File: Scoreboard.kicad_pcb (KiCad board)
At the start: 2 copper layers, 140.5 x 64.5 mm, 256 parts, among them J1 TC2050-IDC-NL, P1 USB_C_Plug_USB2.0, Q1 HL-2301V, Q10 HL-2302V, Q11 HL-2302V, Q12 HL-2302V, Q13 HL-2302V, Q14 HL-2302V, Q15 HL-2302V, Q16 HL-2302V, Q17 HL-2302V, Q18 HL-2302V, Q19 HL-2302V, Q2 HL-2301V, Q20 HL-2302V, Q21 HL-2302V, Q22 HL-2302V, Q23 HL-2302V, Q24 HL-2302V, Q25 HL-2302V, Q3 HL-2301V, Q4 HL-2301V, Q5 HL-2301V, Q6 HL-2301V, Q7 HL-2301V, Q8 HL-2302V, Q9 HL-2302V, SW2 SW_Push, SW3 SW_Push, SW4 SW_Push, U1 AP63203WU, U2 BM832, U3 LM66100DCKR, U4 LM66100DCKR

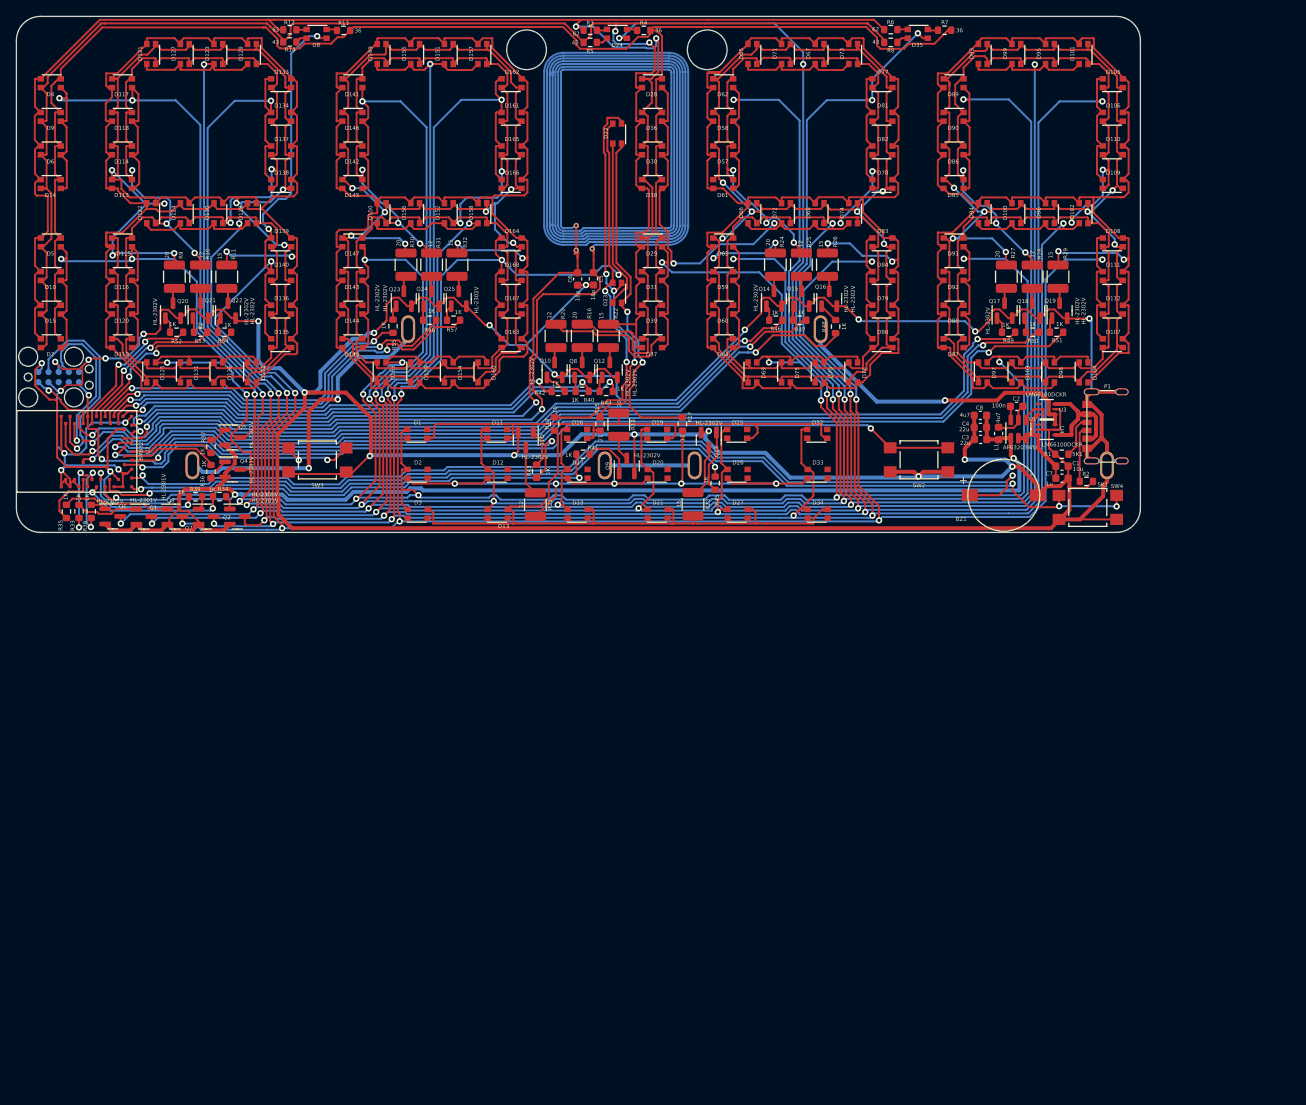
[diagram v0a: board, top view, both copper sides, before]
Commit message: Made a new hardware revision
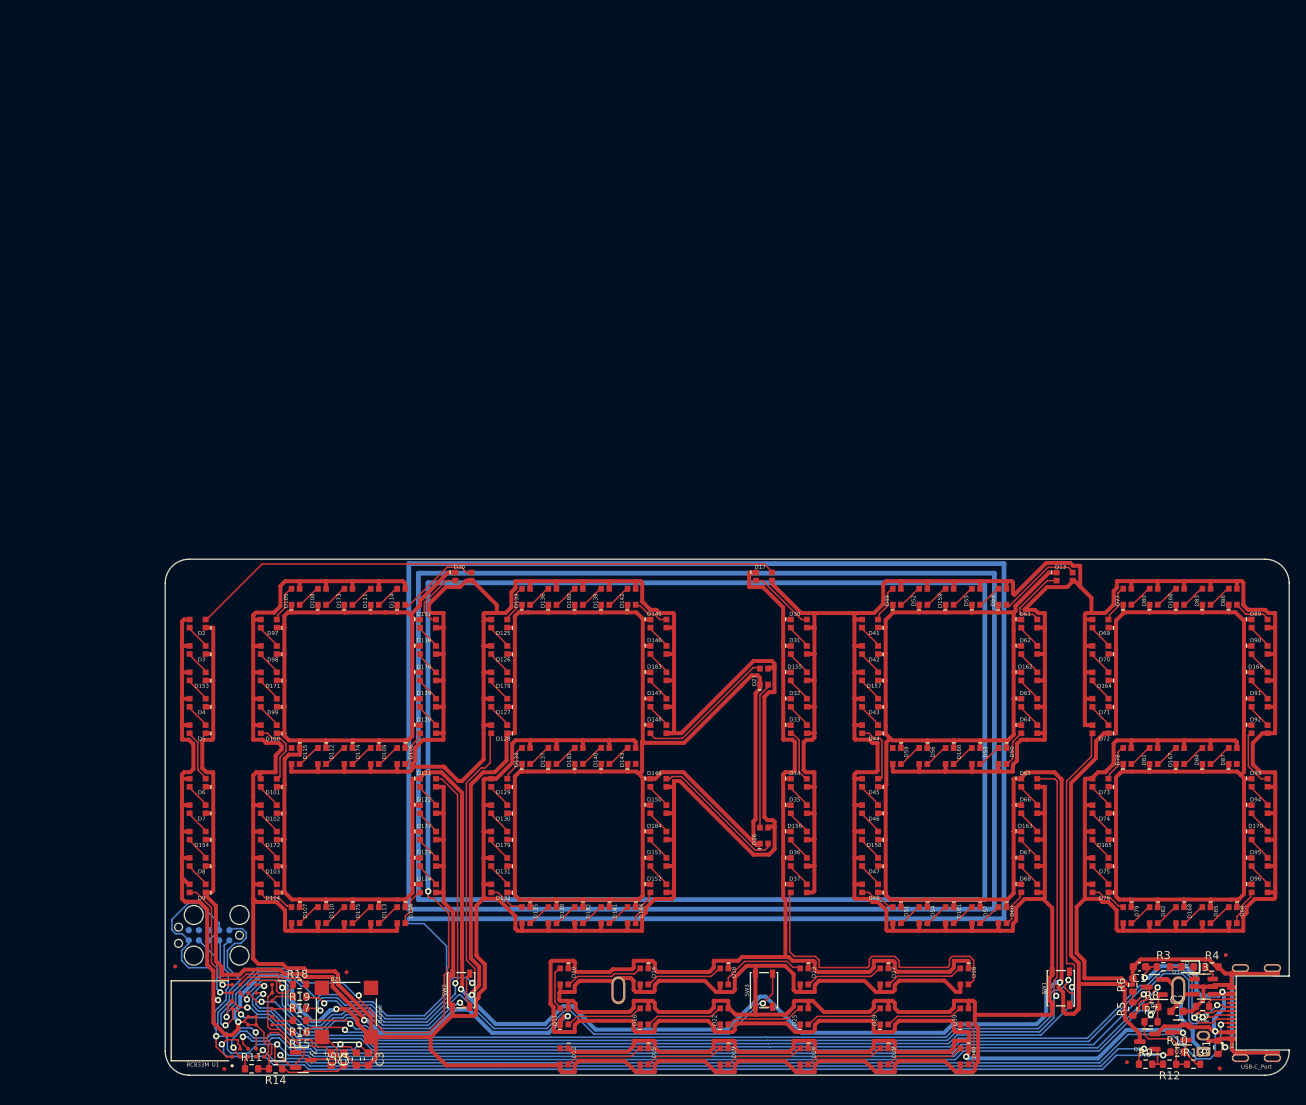
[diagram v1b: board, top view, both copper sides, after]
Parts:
- removed BT3: AA_BATTERY, User_Footprints:BAT_BCAAPC
- removed the C2 at (191.0, 78.2)
- removed C7: 1u, Capacitor_SMD:C_0603_1608Metric
- removed C8: 4u7, Capacitor_SMD:C_0603_1608Metric
- removed the D12 at (126.2, 86.6)
- removed the D30 at (145.4, 46.1)
- removed the D6 at (70.3, 46.1)
- removed L1: 4u7, Inductor_SMD:L_0603_1608Metric
- removed P1: USB_C_Plug_USB2.0, User_Footprints:DEALON_USB-TYPE-C-009
- removed Q10, Q11, Q12, Q13, Q14, Q15, Q16, Q17, Q18, Q19, Q20, Q21, Q22, Q23, Q24, Q25, Q8, Q9: HL-2302V, Package_TO_SOT_SMD:SOT-23
- removed Q5, Q6, Q7: HL-2301V, Package_TO_SOT_SMD:SOT-23
- removed R20, R21, R25, R28, R31: 12, Resistor_SMD:R_1210_3225Metric
- removed R22, R23, R26, R29, R32: 15, Resistor_SMD:R_1210_3225Metric
- removed R24, R27, R30: 20, Resistor_SMD:R_1210_3225Metric
- removed R33, R34, R35, R36, R37, R38, R39, R40, R41, R42, R43, R44, R45, R46, R47, R48, R49, R50, R51, R52, R53, R54, R55, R56, R57: 1K, Resistor_SMD:R_0603_1608Metric
- removed SW4: SW_Push, User_Footprints:SW_SPST_TSC015A03526A
- removed U2: BM832, User_Footprints:BM832
- removed U3, U4: LM66100DCKR, User_Footprints:DCK6_TEX-L
- added D169: LED_WS2812B, User_Footprints:LED_WS2812B_2x1.8mm, F.Cu at (221.4, 111.9)
- added D170: LED_WS2812B, User_Footprints:LED_WS2812B_2x1.8mm, F.Cu at (221.4, 131.8)
- added D171: LED_WS2812B, User_Footprints:LED_WS2812B_2x1.8mm, F.Cu at (97.5, 111.9)
- added D172: LED_WS2812B, User_Footprints:LED_WS2812B_2x1.8mm, F.Cu at (97.5, 131.8)
- added D173: LED_WS2812B, User_Footprints:LED_WS2812B_2x1.8mm, F.Cu at (107.5, 102.0)
- added D174: LED_WS2812B, User_Footprints:LED_WS2812B_2x1.8mm, F.Cu at (107.5, 121.8)
- added D175: LED_WS2812B, User_Footprints:LED_WS2812B_2x1.8mm, F.Cu at (107.5, 141.7)
- added D176: LED_WS2812B, User_Footprints:LED_WS2812B_2x1.8mm, F.Cu at (117.4, 111.9)
- added D177: LED_WS2812B, User_Footprints:LED_WS2812B_2x1.8mm, F.Cu at (117.5, 131.8)
- added D178: LED_WS2812B, User_Footprints:LED_WS2812B_2x1.8mm, F.Cu at (126.4, 111.9)
- added D179: LED_WS2812B, User_Footprints:LED_WS2812B_2x1.8mm, F.Cu at (126.4, 131.8)
- added D180: LED_WS2812B, User_Footprints:LED_WS2812B_2x1.8mm, F.Cu at (136.3, 102.0)
- added D181: LED_WS2812B, User_Footprints:LED_WS2812B_2x1.8mm, F.Cu at (136.3, 121.8)
- added D182: LED_WS2812B, User_Footprints:LED_WS2812B_2x1.8mm, F.Cu at (136.3, 141.7)
- added D183: LED_WS2812B, User_Footprints:LED_WS2812B_2x1.8mm, F.Cu at (146.3, 111.9)
- added D184: LED_WS2812B, User_Footprints:LED_WS2812B_2x1.8mm, F.Cu at (146.2, 131.8)
- added D37: LED_WS2812B, User_Footprints:LED_WS2812B_2x1.8mm, F.Cu at (163.8, 138.4)
- added D40: LED_WS2812B, User_Footprints:LED_WS2812B_2x1.8mm, F.Cu at (184.5, 159.4)
- added D41: LED_WS2812B, User_Footprints:LED_WS2812B_2x1.8mm, F.Cu at (172.7, 105.3)
- added D42: LED_WS2812B, User_Footprints:LED_WS2812B_2x1.8mm, F.Cu at (172.7, 108.6)
- added D43: LED_WS2812B, User_Footprints:LED_WS2812B_2x1.8mm, F.Cu at (172.7, 115.2)
- added D44: LED_WS2812B, User_Footprints:LED_WS2812B_2x1.8mm, F.Cu at (172.7, 118.5)
- added D45: LED_WS2812B, User_Footprints:LED_WS2812B_2x1.8mm, F.Cu at (172.7, 125.2)
- added D46: LED_WS2812B, User_Footprints:LED_WS2812B_2x1.8mm, F.Cu at (172.7, 128.5)
- added D47: LED_WS2812B, User_Footprints:LED_WS2812B_2x1.8mm, F.Cu at (172.7, 135.1)
- added D48: LED_WS2812B, User_Footprints:LED_WS2812B_2x1.8mm, F.Cu at (172.7, 138.4)
- added D49: LED_WS2812B, User_Footprints:LED_WS2812B_2x1.8mm, F.Cu at (176.1, 101.9)
- added D50: LED_WS2812B, User_Footprints:LED_WS2812B_2x1.8mm, F.Cu at (189.2, 121.8)
- added D51: LED_WS2812B, User_Footprints:LED_WS2812B_2x1.8mm, F.Cu at (176.1, 141.7)
- added D52: LED_WS2812B, User_Footprints:LED_WS2812B_2x1.8mm, F.Cu at (179.4, 101.9)
- added D53: LED_WS2812B, User_Footprints:LED_WS2812B_2x1.8mm, F.Cu at (185.9, 121.8)
- added D54: LED_WS2812B, User_Footprints:LED_WS2812B_2x1.8mm, F.Cu at (179.4, 141.7)
- added D55: LED_WS2812B, User_Footprints:LED_WS2812B_2x1.8mm, F.Cu at (186.0, 101.9)
- added D56: LED_WS2812B, User_Footprints:LED_WS2812B_2x1.8mm, F.Cu at (179.3, 121.8)
- added D62: LED_WS2812B, User_Footprints:LED_WS2812B_2x1.8mm, F.Cu at (192.6, 108.6)
- added D69: LED_WS2812B, User_Footprints:LED_WS2812B_2x1.8mm, F.Cu at (201.5, 105.3)
- added D90: LED_WS2812B, User_Footprints:LED_WS2812B_2x1.8mm, F.Cu at (221.4, 108.6)
- added J2: USB-C_Port, User_Footprints:GCT_USB4110GFA, F.Cu at (219.0, 154.0)
- added J3: TP4057, User_Footprints:SOT-23-6, F.Cu at (214.4, 150.7)
- added REF**: Fiducial_0.5mm_Mask1mm, Fiducial:Fiducial_0.5mm_Mask1mm, F.Cu at (92.0, 161.0)
- added REF**: Fiducial_0.5mm_Mask1mm, Fiducial:Fiducial_0.5mm_Mask1mm, F.Cu at (85.8, 148.2)
- added REF**: Fiducial_0.5mm_Mask1mm, Fiducial:Fiducial_0.5mm_Mask1mm, F.Cu at (204.8, 160.1)
- added REF**: Fiducial_0.5mm_Mask1mm, Fiducial:Fiducial_0.5mm_Mask1mm, F.Cu at (107.3, 148.9)
- added REF**: Fiducial_0.5mm_Mask1mm, Fiducial:Fiducial_0.5mm_Mask1mm, F.Cu at (216.4, 160.9)
- added REF**: Fiducial_0.5mm_Mask1mm, Fiducial:Fiducial_0.5mm_Mask1mm, F.Cu at (217.2, 146.7)
- added SW1: SW_Push, User_Footprints:Oval_Button, F.Cu at (196.6, 150.9)
- AE1: footprint User_Footprints:HM-NFC-Class6-Antenna -> User_Footprints:HM-NFC-Class3-Antenna
- BT1: value AA_BATTERY -> LiPo; footprint User_Footprints:BAT_BCAAPC -> User_Footprints:JST_PH_S2B-PH-K_1x02_P2.00mm_Horizontal
- BT2: value AA_BATTERY -> 18650_Cell; footprint User_Footprints:BAT_BCAAPC -> User_Footprints:18650_Cell_Holder
- BZ1: value HYG-9032A -> Buzzer; footprint User_Footprints:MagneticBuzzer_HYG-9032A -> User_Footprints:XDCR_CMT-7525-80-SMT-TR
- C1: value 10u -> 1u; footprint Capacitor_SMD:C_0603_1608Metric -> User_Footprints:C_0603_1608Metric
- C2: renamed from D37; value LED_RGAB -> 1u; footprint User_Footprints:RGB_LED_NH-B2020RGBA-HF -> User_Footprints:C_0603_1608Metric
- C3, C4: value 22u -> 18p; footprint Capacitor_SMD:C_0603_1608Metric -> User_Footprints:C_0603_1608Metric
- C5, C6: value 18p -> 4u7; footprint Capacitor_SMD:C_0603_1608Metric -> User_Footprints:C_0603_1608Metric
- D1: value LED_RGAB -> LED; footprint User_Footprints:RGB_LED_NH-B2020RGBA-HF -> LED_SMD:LED_0603_1608Metric
- D10, D100, D101, D102, D103, D104, D105, D106, D107, D108, D109, D11, D110, D111, D112, D113, D114, D115, D116, D117, D118, D119, D120, D121, D122, D123, D124, D125, D126, D127, D128, D129, D13, D130, D131, D132, D133, D134, D135, D136, D137, D138, D139, D14, D140, D141, D142, D143, D144, D145, D146, D147, D148, D149, D15, D150, D151, D152, D153, D154, D155, D156, D157, D158, D159, D16, D160, D161, D162, D163, D164, D165, D166, D167, D168, D17, D18, D19, D2, D20, D21, D22, D23, D24, D25, D26, D27, D28, D29, D3, D31, D32, D33, D34, D35, D36, D38, D39, D4, D5, D57, D58, D59, D60, D61, D63, D64, D65, D66, D67, D68, D7, D70, D71, D72, D73, D74, D75, D76, D77, D78, D79, D8, D80, D81, D82, D83, D84, D85, D86, D87, D88, D89, D9, D91, D92, D93, D94, D95, D96, D97, D98, D99: value LED_RGAB -> LED_WS2812B; footprint User_Footprints:RGB_LED_NH-B2020RGBA-HF -> User_Footprints:LED_WS2812B_2x1.8mm
- D12: renamed from D69; value LED_RGAB -> LED_WS2812B; footprint User_Footprints:RGB_LED_NH-B2020RGBA-HF -> User_Footprints:LED_WS2812B_2x1.8mm
- D30: renamed from D90; value LED_RGAB -> LED_WS2812B; footprint User_Footprints:RGB_LED_NH-B2020RGBA-HF -> User_Footprints:LED_WS2812B_2x1.8mm
- D6: renamed from D62; value LED_RGAB -> LED_WS2812B; footprint User_Footprints:RGB_LED_NH-B2020RGBA-HF -> User_Footprints:LED_WS2812B_2x1.8mm
- Q1, Q2, Q3, Q4: footprint Package_TO_SOT_SMD:SOT-23 -> User_Footprints:SOT-23
- R1, R2: footprint Resistor_SMD:R_0603_1608Metric -> User_Footprints:R_0603_1608Metric
- R10: value 12 -> 1K; footprint Resistor_SMD:R_1210_3225Metric -> User_Footprints:R_0603_1608Metric
- R11: value 15 -> 1K; footprint Resistor_SMD:R_1210_3225Metric -> User_Footprints:R_0603_1608Metric
- R12: value 62 -> 100K; footprint Resistor_SMD:R_0603_1608Metric -> User_Footprints:R_0603_1608Metric
- R13, R7: value 36 -> 100K; footprint Resistor_SMD:R_0603_1608Metric -> User_Footprints:R_0603_1608Metric
- R14: value 43 -> 100K; footprint Resistor_SMD:R_0603_1608Metric -> User_Footprints:R_0603_1608Metric
- R15: value 21 -> 1K; footprint Resistor_SMD:R_0603_1608Metric -> User_Footprints:R_0603_1608Metric
- R16, R18, R9: value 20 -> 1K; footprint Resistor_SMD:R_1210_3225Metric -> User_Footprints:R_0603_1608Metric
- R17: value 12 -> 1K; footprint Resistor_SMD:R_0603_1608Metric -> User_Footprints:R_0603_1608Metric
- R19: value 15 -> 1K; footprint Resistor_SMD:R_0603_1608Metric -> User_Footprints:R_0603_1608Metric
- R3: value 62 -> 1K; footprint Resistor_SMD:R_0603_1608Metric -> User_Footprints:R_0603_1608Metric
- R4: value 36 -> 1K6; footprint Resistor_SMD:R_0603_1608Metric -> User_Footprints:R_0603_1608Metric
- R5: value 43 -> 5K1; footprint Resistor_SMD:R_0603_1608Metric -> User_Footprints:R_0603_1608Metric
- R6: value 62 -> 5K1; footprint Resistor_SMD:R_0603_1608Metric -> User_Footprints:R_0603_1608Metric
- R8: value 43 -> 1K; footprint Resistor_SMD:R_0603_1608Metric -> User_Footprints:R_0603_1608Metric
- SW2, SW3: footprint User_Footprints:SW_SPST_TSC015A03526A -> User_Footprints:Oval_Button
- U1: value AP63203WU -> BC833M; footprint Package_TO_SOT_SMD:TSOT-23-6 -> User_Footprints:XCVR_BC833M
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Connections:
- BZ1 pad 1: Net-(U2-PadP$17) -> Net-(BZ1-Pad1)
- C1 pad 1: Net-(C1-Pad1) -> VBUS
- C2 pad 1: RED_BOTT_2 -> VBAT
- C2 pad 2: GREEN_BOTT_2 -> GND
- C3 pad 1: +3V3 -> Net-(AE1-Pad1)
- C4 pad 1: +3V3 -> GND
- C4 pad 2: GND -> Net-(AE1-Pad2)
- C5 pad 1: GND -> VBUS
- C5 pad 2: Net-(AE1-Pad2) -> GND
- C6 pad 1: Net-(AE1-Pad1) -> VDD
- D1 pad 1: RED_BOTT_1 -> Net-(D1-Pad1)
- D1 pad 2: unconnected-(D1-Pad2) -> Net-(D1-Pad2)
- D10 pad 1: RED_BOTT_2 -> VLEDS_E
- D10 pad 2: GREEN_BOTT_2 -> Net-(D10-Pad2)
- D10 pad 3: Segment_2-E_OUT -> GND
- D10 pad 4: BLUE_BOTT_2 -> Net-(D10-Pad4)
- D100 pad 1: RED_RIGHT_2 -> VLEDS
- D100 pad 2: GREEN_RIGHT_2 -> Net-(D100-Pad2)
- D100 pad 3: Segment_2-G_OUT -> GND
- D100 pad 4: BLUE_RIGHT_2 -> Net-(D100-Pad4)
- D101 pad 1: RED_RIGHT_2 -> VLEDS
- D101 pad 2: GREEN_RIGHT_2 -> Net-(D100-Pad4)
- D101 pad 3: Segment_2-A_OUT -> GND
- D101 pad 4: BLUE_RIGHT_2 -> Net-(D101-Pad4)
- D102 pad 1: RED_RIGHT_2 -> VLEDS
- D102 pad 2: GREEN_RIGHT_2 -> Net-(D101-Pad4)
- D102 pad 3: Segment_2-G_OUT -> GND
- D102 pad 4: BLUE_RIGHT_2 -> Net-(D102-Pad4)
- D103 pad 1: RED_RIGHT_2 -> VLEDS
- D103 pad 2: GREEN_RIGHT_2 -> Net-(D103-Pad2)
- D103 pad 3: Segment_2-D_OUT -> GND
- D103 pad 4: BLUE_RIGHT_2 -> Net-(D103-Pad4)
- D104 pad 1: RED_RIGHT_2 -> VLEDS
- D104 pad 2: GREEN_RIGHT_2 -> Net-(D103-Pad4)
- D104 pad 3: Segment_2-D_OUT -> GND
- D104 pad 4: BLUE_RIGHT_2 -> Net-(D104-Pad4)
- D105 pad 1: RED_RIGHT_2 -> VLEDS
- D105 pad 2: GREEN_RIGHT_2 -> Net-(D105-Pad2)
- D105 pad 3: Segment_2-B_OUT -> GND
- D105 pad 4: BLUE_RIGHT_2 -> Net-(D105-Pad4)
- D106 pad 1: RED_RIGHT_2 -> VLEDS
- D106 pad 2: GREEN_RIGHT_2 -> Net-(D106-Pad2)
- D106 pad 3: Segment_2-B_OUT -> GND
- D106 pad 4: BLUE_RIGHT_2 -> Net-(D106-Pad4)
- D107 pad 1: RED_RIGHT_2 -> VLEDS
- D107 pad 2: GREEN_RIGHT_2 -> Net-(D104-Pad4)
- D107 pad 3: Segment_2-C_OUT -> GND
- D107 pad 4: BLUE_RIGHT_2 -> Net-(D107-Pad4)
- D108 pad 1: RED_RIGHT_2 -> VLEDS
- D108 pad 2: GREEN_RIGHT_2 -> Net-(D108-Pad2)
- D108 pad 3: Segment_2-C_OUT -> GND
- D108 pad 4: BLUE_RIGHT_2 -> Net-(D105-Pad2)
- D109 pad 1: RED_RIGHT_2 -> VLEDS
- D109 pad 2: GREEN_RIGHT_2 -> Net-(D109-Pad2)
- D109 pad 3: Segment_2-B_OUT -> GND
- D109 pad 4: BLUE_RIGHT_2 -> Net-(D106-Pad2)
- D11 pad 1: RED_BOTT_1 -> VLEDS_E
- D11 pad 2: unconnected-(D11-Pad2) -> Net-(D11-Pad2)
- D11 pad 3: Segment_2-E_OUT -> GND
- D11 pad 4: unconnected-(D11-Pad4) -> Net-(D10-Pad2)
- D110 pad 1: RED_RIGHT_2 -> VLEDS
- D110 pad 2: GREEN_RIGHT_2 -> Net-(D107-Pad4)
- D110 pad 3: Segment_2-B_OUT -> GND
- D110 pad 4: BLUE_RIGHT_2 -> Net-(D110-Pad4)
- D111 pad 1: RED_RIGHT_2 -> VLEDS
- D111 pad 2: GREEN_RIGHT_2 -> Net-(D111-Pad2)
- D111 pad 3: Segment_2-C_OUT -> GND
- D111 pad 4: BLUE_RIGHT_2 -> Net-(D111-Pad4)
- D112 pad 1: RED_RIGHT_2 -> VLEDS
- D112 pad 2: GREEN_RIGHT_2 -> Net-(D112-Pad2)
- D112 pad 3: Segment_2-C_OUT -> GND
- D112 pad 4: BLUE_RIGHT_2 -> Net-(D112-Pad4)
- D113 pad 1: RED_LEFT_1 -> VLEDS
- D113 pad 2: GREEN_LEFT_1 -> Net-(D113-Pad2)
- D113 pad 3: Segment_2-F_OUT -> GND
- D113 pad 4: BLUE_LEFT_1 -> Net-(D113-Pad4)
- D114 pad 1: RED_LEFT_1 -> VLEDS
- D114 pad 2: GREEN_LEFT_1 -> Net-(D114-Pad2)
- D114 pad 3: Segment_2-F_OUT -> GND
- D114 pad 4: BLUE_LEFT_1 -> Net-(D111-Pad2)
- D115 pad 1: RED_LEFT_1 -> VLEDS
- D115 pad 2: GREEN_LEFT_1 -> unconnected-(D115-Pad2)
- D115 pad 3: Segment_2-E_OUT -> GND
- D115 pad 4: BLUE_LEFT_1 -> Net-(D112-Pad2)
- D116 pad 1: RED_LEFT_1 -> VLEDS
- D116 pad 2: GREEN_LEFT_1 -> Net-(D113-Pad4)
- D116 pad 3: Segment_2-E_OUT -> GND
- D116 pad 4: BLUE_LEFT_1 -> Net-(D116-Pad4)
- D117 pad 1: RED_LEFT_1 -> VLEDS
- D117 pad 2: GREEN_LEFT_1 -> Net-(D117-Pad2)
- D117 pad 3: Segment_2-F_OUT -> GND
- D117 pad 4: BLUE_LEFT_1 -> Net-(D117-Pad4)
- D118 pad 1: RED_LEFT_1 -> VLEDS
- D118 pad 2: GREEN_LEFT_1 -> Net-(D118-Pad2)
- D118 pad 3: Segment_2-F_OUT -> GND
- D118 pad 4: BLUE_LEFT_1 -> Net-(D117-Pad2)
- D119 pad 1: RED_LEFT_1 -> VLEDS
- D119 pad 2: GREEN_LEFT_1 -> Net-(D119-Pad2)
- D119 pad 3: Segment_2-E_OUT -> GND
- D119 pad 4: BLUE_LEFT_1 -> Net-(D119-Pad4)
- D12 pad 1: RED_RIGHT_1 -> VLEDS_E
- D12 pad 2: GREEN_RIGHT_1 -> unconnected-(D12-Pad2)
- D12 pad 3: Segment_2-D_OUT -> GND
- D12 pad 4: BLUE_RIGHT_1 -> Net-(D12-Pad4)
- D120 pad 1: RED_LEFT_1 -> VLEDS
- D120 pad 2: GREEN_LEFT_1 -> Net-(D106-Pad4)
- D120 pad 3: Segment_2-E_OUT -> GND
- D120 pad 4: BLUE_LEFT_1 -> Net-(D119-Pad2)
- D121 pad 1: RED_LEFT_1 -> VLEDS
- D121 pad 2: GREEN_LEFT_1 -> Net-(D121-Pad2)
- D121 pad 3: Segment_2-A_OUT -> GND
- D121 pad 4: BLUE_LEFT_1 -> L1_Data
- D122 pad 1: RED_LEFT_1 -> VLEDS
- D122 pad 2: GREEN_LEFT_1 -> Net-(D122-Pad2)
- D122 pad 3: Segment_2-G_OUT -> GND
- D122 pad 4: BLUE_LEFT_1 -> Net-(D121-Pad2)
- D123 pad 1: RED_LEFT_1 -> VLEDS
- D123 pad 2: GREEN_LEFT_1 -> Net-(D123-Pad2)
- D123 pad 3: Segment_2-A_OUT -> GND
- D123 pad 4: BLUE_LEFT_1 -> Net-(D123-Pad4)
- D124 pad 1: RED_LEFT_1 -> VLEDS
- D124 pad 2: GREEN_LEFT_1 -> Net-(D116-Pad4)
- D124 pad 3: Segment_2-G_OUT -> GND
- D124 pad 4: BLUE_LEFT_1 -> Net-(D123-Pad2)
- D125 pad 1: RED_LEFT_1 -> VLEDS
- D125 pad 2: GREEN_LEFT_1 -> Net-(D125-Pad2)
- D125 pad 3: Segment_2-D_OUT -> GND
- D125 pad 4: BLUE_LEFT_1 -> Net-(D125-Pad4)
- D126 pad 1: RED_LEFT_1 -> VLEDS
- D126 pad 2: GREEN_LEFT_1 -> Net-(D125-Pad4)
- D126 pad 3: Segment_2-D_OUT -> GND
- D126 pad 4: BLUE_LEFT_1 -> Net-(D126-Pad4)
- D127 pad 1: RED_LEFT_1 -> VLEDS
- D127 pad 2: GREEN_LEFT_1 -> Net-(D127-Pad2)
- D127 pad 3: Segment_2-A_OUT -> GND
- D127 pad 4: BLUE_LEFT_1 -> Net-(D127-Pad4)
- D128 pad 1: RED_LEFT_1 -> VLEDS
- D128 pad 2: GREEN_LEFT_1 -> Net-(D127-Pad4)
- D128 pad 3: Segment_2-G_OUT -> GND
- D128 pad 4: BLUE_LEFT_1 -> L2_Data
- D129 pad 1: RED_LEFT_1 -> VLEDS
- D129 pad 2: GREEN_LEFT_1 -> Net-(D129-Pad2)
- D129 pad 3: Segment_2-A_OUT -> GND
- D129 pad 4: BLUE_LEFT_1 -> Net-(D129-Pad4)
- D13 pad 1: unconnected-(D13-Pad1) -> VLEDS
- D13 pad 2: unconnected-(D13-Pad2) -> Net-(D13-Pad2)
- D13 pad 3: Segment_2-E_OUT -> GND
- D13 pad 4: BLUE_BOTT_1 -> Net-(D13-Pad4)
- D130 pad 1: RED_LEFT_1 -> VLEDS
- D130 pad 2: GREEN_LEFT_1 -> Net-(D129-Pad4)
- D130 pad 3: Segment_2-G_OUT -> GND
- D130 pad 4: BLUE_LEFT_1 -> Net-(D130-Pad4)
- D131 pad 1: RED_LEFT_1 -> VLEDS
- D131 pad 2: GREEN_LEFT_1 -> Net-(D131-Pad2)
- D131 pad 3: Segment_2-D_OUT -> GND
- D131 pad 4: BLUE_LEFT_1 -> Net-(D131-Pad4)
- D132 pad 1: RED_LEFT_1 -> VLEDS
- D132 pad 2: GREEN_LEFT_1 -> Net-(D131-Pad4)
- D132 pad 3: Segment_2-D_OUT -> GND
- D132 pad 4: BLUE_LEFT_1 -> Net-(D132-Pad4)
- D133 pad 1: RED_LEFT_1 -> VLEDS
- D133 pad 2: GREEN_LEFT_1 -> Net-(D133-Pad2)
- D133 pad 3: Segment_2-B_OUT -> GND
- D133 pad 4: BLUE_LEFT_1 -> Net-(D125-Pad2)
- D134 pad 1: RED_LEFT_1 -> VLEDS
- D134 pad 2: GREEN_LEFT_1 -> Net-(D134-Pad2)
- D134 pad 3: Segment_2-B_OUT -> GND
- D134 pad 4: BLUE_LEFT_1 -> Net-(D129-Pad2)
- D135 pad 1: RED_LEFT_1 -> VLEDS
- D135 pad 2: GREEN_LEFT_1 -> Net-(D132-Pad4)
- D135 pad 3: Segment_2-C_OUT -> GND
- D135 pad 4: BLUE_LEFT_1 -> Net-(D135-Pad4)
- D136 pad 1: RED_LEFT_1 -> VLEDS
- D136 pad 2: GREEN_LEFT_1 -> Net-(D136-Pad2)
- D136 pad 3: Segment_2-C_OUT -> GND
- D136 pad 4: BLUE_LEFT_1 -> Net-(D133-Pad2)
- D137 pad 1: RED_LEFT_1 -> VLEDS
- D137 pad 2: GREEN_LEFT_1 -> Net-(D137-Pad2)
- D137 pad 3: Segment_2-B_OUT -> GND
- D137 pad 4: BLUE_LEFT_1 -> Net-(D134-Pad2)
- D138 pad 1: RED_LEFT_1 -> VLEDS
- D138 pad 2: GREEN_LEFT_1 -> Net-(D135-Pad4)
- D138 pad 3: Segment_2-B_OUT -> GND
- D138 pad 4: BLUE_LEFT_1 -> Net-(D138-Pad4)
- D139 pad 1: RED_LEFT_1 -> VLEDS
- D139 pad 2: GREEN_LEFT_1 -> Net-(D139-Pad2)
- D139 pad 3: Segment_2-C_OUT -> GND
- D139 pad 4: BLUE_LEFT_1 -> Net-(D139-Pad4)
- D14 pad 1: RED_BOTT_2 -> VLEDS_E
- D14 pad 2: GREEN_BOTT_2 -> Net-(D10-Pad4)
- D14 pad 3: Segment_2-F_OUT -> GND
- D14 pad 4: BLUE_BOTT_2 -> Net-(D14-Pad4)
- D140 pad 1: RED_LEFT_1 -> VLEDS
- D140 pad 2: GREEN_LEFT_1 -> Net-(D140-Pad2)
- D140 pad 3: Segment_2-C_OUT -> GND
- D140 pad 4: BLUE_LEFT_1 -> Net-(D140-Pad4)
- D141 pad 1: RED_LEFT_2 -> VLEDS
- D141 pad 2: GREEN_LEFT_2 -> Net-(D141-Pad2)
- D141 pad 3: Segment_2-F_OUT -> GND
- D141 pad 4: BLUE_LEFT_2 -> Net-(D141-Pad4)
- D142 pad 1: RED_LEFT_2 -> VLEDS
- D142 pad 2: GREEN_LEFT_2 -> Net-(D142-Pad2)
- D142 pad 3: Segment_2-F_OUT -> GND
- D142 pad 4: BLUE_LEFT_2 -> Net-(D139-Pad2)
- D143 pad 1: RED_LEFT_2 -> VLEDS
- D143 pad 2: GREEN_LEFT_2 -> unconnected-(D143-Pad2)
- D143 pad 3: Segment_2-E_OUT -> GND
- D143 pad 4: BLUE_LEFT_2 -> Net-(D140-Pad2)
- D144 pad 1: RED_LEFT_2 -> VLEDS
- D144 pad 2: GREEN_LEFT_2 -> Net-(D141-Pad4)
- D144 pad 3: Segment_2-E_OUT -> GND
- D144 pad 4: BLUE_LEFT_2 -> Net-(D144-Pad4)
- D145 pad 1: RED_LEFT_2 -> VLEDS
- D145 pad 2: GREEN_LEFT_2 -> Net-(D145-Pad2)
- D145 pad 3: Segment_2-F_OUT -> GND
- D145 pad 4: BLUE_LEFT_2 -> Net-(D142-Pad2)
- D146 pad 1: RED_LEFT_2 -> VLEDS
- D146 pad 2: GREEN_LEFT_2 -> Net-(D146-Pad2)
- D146 pad 3: Segment_2-F_OUT -> GND
- D146 pad 4: BLUE_LEFT_2 -> Net-(D145-Pad2)
- D147 pad 1: RED_LEFT_2 -> VLEDS
- D147 pad 2: GREEN_LEFT_2 -> Net-(D147-Pad2)
- D147 pad 3: Segment_2-E_OUT -> GND
- D147 pad 4: BLUE_LEFT_2 -> Net-(D147-Pad4)
- D148 pad 1: RED_LEFT_2 -> VLEDS
- D148 pad 2: GREEN_LEFT_2 -> Net-(D148-Pad2)
- D148 pad 3: Segment_2-E_OUT -> GND
- D148 pad 4: BLUE_LEFT_2 -> Net-(D147-Pad2)
- D149 pad 1: RED_LEFT_2 -> VLEDS
- D149 pad 2: GREEN_LEFT_2 -> Net-(D149-Pad2)
- D149 pad 3: Segment_2-A_OUT -> GND
- D149 pad 4: BLUE_LEFT_2 -> Net-(D149-Pad4)
- D15 pad 1: RED_BOTT_2 -> VLEDS_E
- D15 pad 2: GREEN_BOTT_2 -> Net-(D12-Pad4)
- D15 pad 3: Segment_2-E_OUT -> GND
- D15 pad 4: BLUE_BOTT_2 -> Net-(D15-Pad4)
- D150 pad 1: RED_LEFT_2 -> VLEDS
- D150 pad 2: GREEN_LEFT_2 -> Net-(D150-Pad2)
- D150 pad 3: Segment_2-G_OUT -> GND
- D150 pad 4: BLUE_LEFT_2 -> Net-(D149-Pad2)
- D151 pad 1: RED_LEFT_2 -> VLEDS
- D151 pad 2: GREEN_LEFT_2 -> Net-(D151-Pad2)
- D151 pad 3: Segment_2-A_OUT -> GND
- D151 pad 4: BLUE_LEFT_2 -> Net-(D151-Pad4)
- D152 pad 1: RED_LEFT_2 -> VLEDS
- D152 pad 2: GREEN_LEFT_2 -> Net-(D144-Pad4)
- D152 pad 3: Segment_2-G_OUT -> GND
- D152 pad 4: BLUE_LEFT_2 -> Net-(D151-Pad2)
- D153 pad 1: RED_LEFT_2 -> VLEDS_E
- D153 pad 2: GREEN_LEFT_2 -> Net-(D153-Pad2)
- D153 pad 3: Segment_2-D_OUT -> GND
- D153 pad 4: BLUE_LEFT_2 -> Net-(D153-Pad4)
- D154 pad 1: RED_LEFT_2 -> VLEDS_E
- D154 pad 2: GREEN_LEFT_2 -> Net-(D154-Pad2)
- D154 pad 3: Segment_2-D_OUT -> GND
- D154 pad 4: BLUE_LEFT_2 -> Net-(D154-Pad4)
- D155 pad 1: RED_LEFT_2 -> VLEDS_E
- D155 pad 2: GREEN_LEFT_2 -> Net-(D155-Pad2)
- D155 pad 3: Segment_2-A_OUT -> GND
- D155 pad 4: BLUE_LEFT_2 -> Net-(D155-Pad4)
- D156 pad 1: RED_LEFT_2 -> VLEDS_E
- D156 pad 2: GREEN_LEFT_2 -> Net-(D156-Pad2)
- D156 pad 3: Segment_2-G_OUT -> GND
- D156 pad 4: BLUE_LEFT_2 -> Net-(D156-Pad4)
- D157 pad 1: RED_LEFT_2 -> VLEDS
- D157 pad 2: GREEN_LEFT_2 -> Net-(D157-Pad2)
- D157 pad 3: Segment_2-A_OUT -> GND
- D157 pad 4: BLUE_LEFT_2 -> Net-(D157-Pad4)
- D158 pad 1: RED_LEFT_2 -> VLEDS
- D158 pad 2: GREEN_LEFT_2 -> Net-(D158-Pad2)
- D158 pad 3: Segment_2-G_OUT -> GND
- D158 pad 4: BLUE_LEFT_2 -> Net-(D158-Pad4)
- D159 pad 1: RED_LEFT_2 -> VLEDS
- D159 pad 2: GREEN_LEFT_2 -> Net-(D159-Pad2)
- D159 pad 3: Segment_2-D_OUT -> GND
- D159 pad 4: BLUE_LEFT_2 -> Net-(D159-Pad4)
- D16 pad 1: RED_BOTT_1 -> VLEDS_E
- D16 pad 2: unconnected-(D16-Pad2) -> Net-(D16-Pad2)
- D16 pad 3: Segment_2-F_OUT -> GND
- D16 pad 4: unconnected-(D16-Pad4) -> Net-(D11-Pad2)
- D160 pad 1: RED_LEFT_2 -> VLEDS
- D160 pad 2: GREEN_LEFT_2 -> Net-(D160-Pad2)
- D160 pad 3: Segment_2-D_OUT -> GND
- D160 pad 4: BLUE_LEFT_2 -> Net-(D160-Pad4)
- D161 pad 1: RED_LEFT_2 -> VLEDS
- D161 pad 2: GREEN_LEFT_2 -> Net-(D161-Pad2)
- D161 pad 3: Segment_2-B_OUT -> GND
- D161 pad 4: BLUE_LEFT_2 -> Net-(D161-Pad4)
- D162 pad 1: RED_LEFT_2 -> VLEDS
- D162 pad 2: GREEN_LEFT_2 -> Net-(D162-Pad2)
- D162 pad 3: Segment_2-B_OUT -> GND
- D162 pad 4: BLUE_LEFT_2 -> Net-(D162-Pad4)
- D163 pad 1: RED_LEFT_2 -> VLEDS
- D163 pad 2: GREEN_LEFT_2 -> Net-(D163-Pad2)
- D163 pad 3: Segment_2-C_OUT -> GND
- D163 pad 4: BLUE_LEFT_2 -> Net-(D163-Pad4)
- D164 pad 1: RED_LEFT_2 -> VLEDS
- D164 pad 2: GREEN_LEFT_2 -> Net-(D164-Pad2)
- D164 pad 3: Segment_2-C_OUT -> GND
- D164 pad 4: BLUE_LEFT_2 -> Net-(D164-Pad4)
- D165 pad 1: RED_LEFT_2 -> VLEDS
- D165 pad 2: GREEN_LEFT_2 -> Net-(D165-Pad2)
- D165 pad 3: Segment_2-B_OUT -> GND
- D165 pad 4: BLUE_LEFT_2 -> Net-(D165-Pad4)
- D166 pad 1: RED_LEFT_2 -> VLEDS
- D166 pad 2: GREEN_LEFT_2 -> Net-(D166-Pad2)
- D166 pad 3: Segment_2-B_OUT -> GND
- D166 pad 4: BLUE_LEFT_2 -> Net-(D166-Pad4)
- D167 pad 1: RED_LEFT_2 -> VLEDS
- D167 pad 2: GREEN_LEFT_2 -> Net-(D167-Pad2)
- D167 pad 3: Segment_2-C_OUT -> GND
- D167 pad 4: BLUE_LEFT_2 -> Net-(D167-Pad4)
- D168 pad 1: RED_LEFT_2 -> VLEDS
- D168 pad 2: GREEN_LEFT_2 -> Net-(D168-Pad2)
- D168 pad 3: Segment_2-C_OUT -> GND
- D168 pad 4: BLUE_LEFT_2 -> Net-(D168-Pad4)
- D17 pad 1: unconnected-(D17-Pad1) -> VLEDS_E
- D17 pad 2: GREEN_BOTT_1 -> Net-(D17-Pad2)
- D17 pad 3: Segment_2-F_OUT -> GND
- D17 pad 4: unconnected-(D17-Pad4) -> Net-(D17-Pad4)
- D18 pad 1: unconnected-(D18-Pad1) -> VLEDS_E
- D18 pad 2: unconnected-(D18-Pad2) -> Net-(D14-Pad4)
- D18 pad 3: Segment_2-F_OUT -> GND
- D18 pad 4: BLUE_BOTT_1 -> Net-(D18-Pad4)
- D19 pad 1: RED_BOTT_1 -> VLEDS_E
- D19 pad 2: unconnected-(D19-Pad2) -> Net-(D15-Pad4)
- D19 pad 3: Segment_2-A_OUT -> GND
- D19 pad 4: unconnected-(D19-Pad4) -> Net-(D19-Pad4)
- D2 pad 1: unconnected-(D2-Pad1) -> VLEDS_E
- D2 pad 2: GREEN_BOTT_1 -> Net-(D17-Pad4)
- D2 pad 3: Segment_2-D_OUT -> GND
- D2 pad 4: unconnected-(D2-Pad4) -> Net-(D2-Pad4)
- D20 pad 1: unconnected-(D20-Pad1) -> VLEDS
- D20 pad 2: GREEN_BOTT_1 -> Net-(D117-Pad4)
- D20 pad 3: Segment_2-A_OUT -> GND
- D20 pad 4: unconnected-(D20-Pad4) -> Net-(D114-Pad2)
- D21 pad 1: unconnected-(D21-Pad1) -> VLEDS
- D21 pad 2: unconnected-(D21-Pad2) -> Net-(D21-Pad2)
- D21 pad 3: Segment_2-A_OUT -> GND
- D21 pad 4: BLUE_BOTT_1 -> Net-(D148-Pad2)
- D22 pad 1: Net-(D22-Pad1) -> VLEDS_E
- D22 pad 3: Segment_2-C_OUT -> GND
- D22 pad 4: Net-(D22-Pad4) -> Net-(D16-Pad2)
- D23 pad 1: Net-(D22-Pad1) -> VLEDS_E
- D23 pad 2: Net-(D22-Pad2) -> Net-(D18-Pad4)
- D23 pad 3: Segment_2-C_OUT -> GND
- D23 pad 4: Net-(D22-Pad4) -> Net-(D23-Pad4)
- D24 pad 1: Net-(D24-Pad1) -> VLEDS_E
- D24 pad 2: Net-(D24-Pad2) -> Net-(D19-Pad4)
- D24 pad 3: Segment_2-A_OUT -> GND
- D25 pad 1: RED_BOTT_1 -> VLEDS_E
- D25 pad 2: unconnected-(D25-Pad2) -> Net-(D25-Pad2)
- D25 pad 3: Segment_2-B_OUT -> GND
- D25 pad 4: unconnected-(D25-Pad4) -> Net-(D22-Pad2)
- D26 pad 1: unconnected-(D26-Pad1) -> VLEDS
- D26 pad 2: GREEN_BOTT_1 -> Net-(D149-Pad4)
- D26 pad 3: Segment_2-B_OUT -> GND
- D26 pad 4: unconnected-(D26-Pad4) -> Net-(D21-Pad2)
- D27 pad 1: unconnected-(D27-Pad1) -> VLEDS_E
- D27 pad 2: unconnected-(D27-Pad2) -> Net-(D23-Pad4)
- D27 pad 3: Segment_2-B_OUT -> GND
- D27 pad 4: BLUE_BOTT_1 -> Net-(D27-Pad4)
- D28 pad 1: RED_BOTT_2 -> VLEDS_E
- D28 pad 2: GREEN_BOTT_2 -> Net-(D24-Pad4)
- D28 pad 3: Segment_2-G_OUT -> GND
- D28 pad 4: BLUE_BOTT_2 -> Net-(D28-Pad4)
- D29 pad 1: RED_BOTT_2 -> VLEDS_E
- D29 pad 2: GREEN_BOTT_2 -> Net-(D29-Pad2)
- D29 pad 3: Segment_2-D_OUT -> GND
- D29 pad 4: BLUE_BOTT_2 -> Net-(D25-Pad2)
- D3 pad 1: unconnected-(D3-Pad1) -> VLEDS_E
- D3 pad 2: unconnected-(D3-Pad2) -> Net-(D2-Pad4)
- D3 pad 3: Segment_2-D_OUT -> GND
- D3 pad 4: BLUE_BOTT_1 -> Net-(D153-Pad2)
- D30 pad 1: RED_RIGHT_2 -> VLEDS_E
- D30 pad 2: GREEN_RIGHT_2 -> Net-(D30-Pad2)
- D30 pad 3: Segment_2-F_OUT -> GND
- D30 pad 4: BLUE_RIGHT_2 -> Net-(D17-Pad2)
- D31 pad 1: RED_BOTT_2 -> VLEDS_E
- D31 pad 2: GREEN_BOTT_2 -> Net-(D155-Pad4)
- D31 pad 3: Segment_2-D_OUT -> GND
- D31 pad 4: BLUE_BOTT_2 -> Net-(D30-Pad2)
- D32 pad 1: RED_BOTT_1 -> VLEDS_E
- D32 pad 2: unconnected-(D32-Pad2) -> Net-(D32-Pad2)
- D32 pad 3: Segment_2-G_OUT -> GND
- D32 pad 4: unconnected-(D32-Pad4) -> Net-(D155-Pad2)
- D33 pad 1: unconnected-(D33-Pad1) -> VLEDS_E
- D33 pad 2: GREEN_BOTT_1 -> Net-(D33-Pad2)
- D33 pad 3: Segment_2-G_OUT -> GND
- D33 pad 4: unconnected-(D33-Pad4) -> Net-(D32-Pad2)
- D34 pad 1: unconnected-(D34-Pad1) -> VLEDS_E
- D34 pad 2: unconnected-(D34-Pad2) -> Net-(D34-Pad2)
- D34 pad 3: Segment_2-G_OUT -> GND
- D34 pad 4: BLUE_BOTT_1 -> Net-(D33-Pad2)
- D35 pad 1: Net-(D35-Pad1) -> VLEDS_E
- D35 pad 2: Net-(D35-Pad2) -> Net-(D156-Pad4)
- D35 pad 3: Segment_2-B_OUT -> GND
- D35 pad 4: Net-(D35-Pad4) -> Net-(D34-Pad2)
- D36 pad 1: RED_BOTT_2 -> VLEDS_E
- D36 pad 2: GREEN_BOTT_2 -> Net-(D36-Pad2)
- D36 pad 3: Segment_2-G_OUT -> GND
- D36 pad 4: BLUE_BOTT_2 -> Net-(D156-Pad2)
- D38 pad 1: RED_BOTT_2 -> VLEDS_E
- D38 pad 2: GREEN_BOTT_2 -> Net-(D27-Pad4)
- D38 pad 3: Segment_2-G_OUT -> GND
- D38 pad 4: BLUE_BOTT_2 -> Net-(D37-Pad2)
- D39 pad 1: RED_BOTT_2 -> VLEDS_E
- D39 pad 2: GREEN_BOTT_2 -> Net-(D39-Pad2)
- D39 pad 3: Segment_2-D_OUT -> GND
- D39 pad 4: BLUE_BOTT_2 -> Net-(D29-Pad2)
- D4 pad 1: RED_BOTT_2 -> VLEDS_E
- D4 pad 2: GREEN_BOTT_2 -> Net-(D153-Pad4)
- D4 pad 3: Segment_2-F_OUT -> GND
- D4 pad 4: BLUE_BOTT_2 -> Net-(D4-Pad4)
- D5 pad 1: RED_BOTT_2 -> VLEDS_E
- D5 pad 2: GREEN_BOTT_2 -> Net-(D4-Pad4)
- D5 pad 3: Segment_2-E_OUT -> GND
- D5 pad 4: BLUE_BOTT_2 -> Net-(D5-Pad4)
- D57 pad 1: RED_RIGHT_1 -> VLEDS
- D57 pad 2: GREEN_RIGHT_1 -> Net-(D161-Pad4)
- D57 pad 3: Segment_2-F_OUT -> GND
- D57 pad 4: BLUE_RIGHT_1 -> Net-(D57-Pad4)
- D58 pad 1: RED_RIGHT_1 -> VLEDS
- D58 pad 2: GREEN_RIGHT_1 -> Net-(D13-Pad4)
- D58 pad 3: Segment_2-F_OUT -> GND
- D58 pad 4: BLUE_RIGHT_1 -> Net-(D55-Pad2)
- D59 pad 1: RED_RIGHT_1 -> VLEDS
- D59 pad 2: GREEN_RIGHT_1 -> unconnected-(D59-Pad2)
- D59 pad 3: Segment_2-E_OUT -> GND
- D59 pad 4: BLUE_RIGHT_1 -> Net-(D56-Pad2)
- D6 pad 1: RED_RIGHT_1 -> VLEDS_E
- D6 pad 2: GREEN_RIGHT_1 -> Net-(D5-Pad4)
- D6 pad 3: Segment_2-F_OUT -> GND
- D6 pad 4: BLUE_RIGHT_1 -> Net-(D6-Pad4)
- D60 pad 1: RED_RIGHT_1 -> VLEDS
- D60 pad 2: GREEN_RIGHT_1 -> Net-(D57-Pad4)
- D60 pad 3: Segment_2-E_OUT -> GND
- D60 pad 4: BLUE_RIGHT_1 -> Net-(D60-Pad4)
- D61 pad 1: RED_RIGHT_1 -> VLEDS
- D61 pad 2: GREEN_RIGHT_1 -> Net-(D61-Pad2)
- D61 pad 3: Segment_2-F_OUT -> GND
- D61 pad 4: BLUE_RIGHT_1 -> Net-(D13-Pad2)
- D63 pad 1: RED_RIGHT_1 -> VLEDS
- D63 pad 2: GREEN_RIGHT_1 -> Net-(D63-Pad2)
- D63 pad 3: Segment_2-E_OUT -> GND
- D63 pad 4: BLUE_RIGHT_1 -> Net-(D162-Pad2)
- D64 pad 1: RED_RIGHT_1 -> VLEDS
- D64 pad 2: GREEN_RIGHT_1 -> Net-(D50-Pad4)
- D64 pad 3: Segment_2-E_OUT -> GND
- D64 pad 4: BLUE_RIGHT_1 -> Net-(D63-Pad2)
- D65 pad 1: RED_RIGHT_1 -> VLEDS
- D65 pad 2: GREEN_RIGHT_1 -> Net-(D65-Pad2)
- D65 pad 3: Segment_2-A_OUT -> GND
- D65 pad 4: BLUE_RIGHT_1 -> R1_Data
- D66 pad 1: RED_RIGHT_1 -> VLEDS
- D66 pad 2: GREEN_RIGHT_1 -> Net-(D163-Pad4)
- D66 pad 3: Segment_2-G_OUT -> GND
- D66 pad 4: BLUE_RIGHT_1 -> Net-(D65-Pad2)
- D67 pad 1: RED_RIGHT_1 -> VLEDS
- D67 pad 2: GREEN_RIGHT_1 -> Net-(D67-Pad2)
- D67 pad 3: Segment_2-A_OUT -> GND
- D67 pad 4: BLUE_RIGHT_1 -> Net-(D163-Pad2)
- D68 pad 1: RED_RIGHT_1 -> VLEDS
- D68 pad 2: GREEN_RIGHT_1 -> Net-(D60-Pad4)
- D68 pad 3: Segment_2-G_OUT -> GND
- D68 pad 4: BLUE_RIGHT_1 -> Net-(D67-Pad2)
- D7 pad 1: RED_BOTT_2 -> VLEDS_E
- D7 pad 2: GREEN_BOTT_2 -> Net-(D6-Pad4)
- D7 pad 3: Segment_2-E_OUT -> GND
- D7 pad 4: BLUE_BOTT_2 -> Net-(D154-Pad2)
- D70 pad 1: RED_RIGHT_1 -> VLEDS
- D70 pad 2: GREEN_RIGHT_1 -> Net-(D69-Pad4)
- D70 pad 3: Segment_2-D_OUT -> GND
- D70 pad 4: BLUE_RIGHT_1 -> Net-(D164-Pad2)
- D71 pad 1: RED_RIGHT_1 -> VLEDS
- D71 pad 2: GREEN_RIGHT_1 -> Net-(D164-Pad4)
- D71 pad 3: Segment_2-A_OUT -> GND
- D71 pad 4: BLUE_RIGHT_1 -> Net-(D71-Pad4)
- D72 pad 1: RED_RIGHT_1 -> VLEDS
- D72 pad 2: GREEN_RIGHT_1 -> Net-(D71-Pad4)
- D72 pad 3: Segment_2-G_OUT -> GND
- D72 pad 4: BLUE_RIGHT_1 -> R2_Data
- D73 pad 1: RED_RIGHT_1 -> VLEDS
- D73 pad 2: GREEN_RIGHT_1 -> Net-(D73-Pad2)
- D73 pad 3: Segment_2-A_OUT -> GND
- D73 pad 4: BLUE_RIGHT_1 -> Net-(D73-Pad4)
- D74 pad 1: RED_RIGHT_1 -> VLEDS
- D74 pad 2: GREEN_RIGHT_1 -> Net-(D73-Pad4)
- D74 pad 3: Segment_2-G_OUT -> GND
- D74 pad 4: BLUE_RIGHT_1 -> Net-(D165-Pad2)
- D75 pad 1: RED_RIGHT_1 -> VLEDS
- D75 pad 2: GREEN_RIGHT_1 -> Net-(D165-Pad4)
- D75 pad 3: Segment_2-D_OUT -> GND
- D75 pad 4: BLUE_RIGHT_1 -> Net-(D75-Pad4)
- D76 pad 1: RED_RIGHT_1 -> VLEDS
- D76 pad 2: GREEN_RIGHT_1 -> Net-(D75-Pad4)
- D76 pad 3: Segment_2-D_OUT -> GND
- D76 pad 4: BLUE_RIGHT_1 -> Net-(D76-Pad4)
- D77 pad 1: RED_RIGHT_1 -> VLEDS
- D77 pad 2: GREEN_RIGHT_1 -> Net-(D77-Pad2)
- D77 pad 3: Segment_2-B_OUT -> GND
- D77 pad 4: BLUE_RIGHT_1 -> Net-(D69-Pad2)
- D78 pad 1: RED_RIGHT_1 -> VLEDS
- D78 pad 2: GREEN_RIGHT_1 -> Net-(D78-Pad2)
- D78 pad 3: Segment_2-B_OUT -> GND
- D78 pad 4: BLUE_RIGHT_1 -> Net-(D73-Pad2)
- D79 pad 1: RED_RIGHT_1 -> VLEDS
- D79 pad 2: GREEN_RIGHT_1 -> Net-(D76-Pad4)
- D79 pad 3: Segment_2-C_OUT -> GND
- D79 pad 4: BLUE_RIGHT_1 -> Net-(D79-Pad4)
- D8 pad 1: Net-(D8-Pad1) -> VLEDS_E
- D8 pad 2: Net-(D8-Pad2) -> Net-(D154-Pad4)
- D8 pad 3: Segment_2-C_OUT -> GND
- D80 pad 1: RED_RIGHT_1 -> VLEDS
- D80 pad 2: GREEN_RIGHT_1 -> Net-(D166-Pad4)
- D80 pad 3: Segment_2-C_OUT -> GND
- D80 pad 4: BLUE_RIGHT_1 -> Net-(D77-Pad2)
- D81 pad 1: RED_RIGHT_1 -> VLEDS
- D81 pad 2: GREEN_RIGHT_1 -> Net-(D167-Pad4)
- D81 pad 3: Segment_2-B_OUT -> GND
- D81 pad 4: BLUE_RIGHT_1 -> Net-(D78-Pad2)
- D82 pad 1: RED_RIGHT_1 -> VLEDS
- D82 pad 2: GREEN_RIGHT_1 -> Net-(D79-Pad4)
- D82 pad 3: Segment_2-B_OUT -> GND
- D82 pad 4: BLUE_RIGHT_1 -> Net-(D168-Pad2)
- D83 pad 1: RED_RIGHT_1 -> VLEDS
- D83 pad 2: GREEN_RIGHT_1 -> Net-(D83-Pad2)
- D83 pad 3: Segment_2-C_OUT -> GND
- D83 pad 4: BLUE_RIGHT_1 -> Net-(D166-Pad2)
- D84 pad 1: RED_RIGHT_1 -> VLEDS
- D84 pad 2: GREEN_RIGHT_1 -> Net-(D84-Pad2)
- D84 pad 3: Segment_2-C_OUT -> GND
- D84 pad 4: BLUE_RIGHT_1 -> Net-(D167-Pad2)
- D85 pad 1: RED_RIGHT_2 -> VLEDS
- D85 pad 2: GREEN_RIGHT_2 -> Net-(D168-Pad4)
- D85 pad 3: Segment_2-F_OUT -> GND
- D85 pad 4: BLUE_RIGHT_2 -> Net-(D85-Pad4)
- D86 pad 1: RED_RIGHT_2 -> VLEDS
- D86 pad 2: GREEN_RIGHT_2 -> Net-(D86-Pad2)
- D86 pad 3: Segment_2-F_OUT -> GND
- D86 pad 4: BLUE_RIGHT_2 -> Net-(D83-Pad2)
- D87 pad 1: RED_RIGHT_2 -> VLEDS
- D87 pad 2: GREEN_RIGHT_2 -> unconnected-(D87-Pad2)
- D87 pad 3: Segment_2-E_OUT -> GND
- D87 pad 4: BLUE_RIGHT_2 -> Net-(D84-Pad2)
- D88 pad 1: RED_RIGHT_2 -> VLEDS
- D88 pad 2: GREEN_RIGHT_2 -> Net-(D85-Pad4)
- D88 pad 3: Segment_2-E_OUT -> GND
- D88 pad 4: BLUE_RIGHT_2 -> Net-(D88-Pad4)
- D89 pad 1: RED_RIGHT_2 -> VLEDS
- D89 pad 2: GREEN_RIGHT_2 -> Net-(D89-Pad2)
- D89 pad 3: Segment_2-F_OUT -> GND
- D89 pad 4: BLUE_RIGHT_2 -> Net-(D86-Pad2)
- D9 pad 1: RED_BOTT_2 -> VLEDS_E
- D9 pad 2: GREEN_BOTT_2 -> Net-(D8-Pad4)
- D9 pad 3: Segment_2-F_OUT -> GND
- D9 pad 4: BLUE_BOTT_2 -> E1_Data
- D91 pad 1: RED_RIGHT_2 -> VLEDS
- D91 pad 2: GREEN_RIGHT_2 -> Net-(D91-Pad2)
- D91 pad 3: Segment_2-E_OUT -> GND
- D91 pad 4: BLUE_RIGHT_2 -> Net-(D169-Pad2)
- D92 pad 1: RED_RIGHT_2 -> VLEDS
- D92 pad 2: GREEN_RIGHT_2 -> Net-(D92-Pad2)
- D92 pad 3: Segment_2-E_OUT -> GND
- D92 pad 4: BLUE_RIGHT_2 -> Net-(D91-Pad2)
- D93 pad 1: RED_RIGHT_2 -> VLEDS
- D93 pad 2: GREEN_RIGHT_2 -> Net-(D93-Pad2)
- D93 pad 3: Segment_2-A_OUT -> GND
- D93 pad 4: BLUE_RIGHT_2 -> Net-(D92-Pad2)
- D94 pad 1: RED_RIGHT_2 -> VLEDS
- D94 pad 2: GREEN_RIGHT_2 -> Net-(D170-Pad4)
- D94 pad 3: Segment_2-G_OUT -> GND
- D94 pad 4: BLUE_RIGHT_2 -> Net-(D93-Pad2)
- D95 pad 1: RED_RIGHT_2 -> VLEDS
- D95 pad 2: GREEN_RIGHT_2 -> Net-(D95-Pad2)
- D95 pad 3: Segment_2-A_OUT -> GND
- D95 pad 4: BLUE_RIGHT_2 -> Net-(D170-Pad2)
- D96 pad 1: RED_RIGHT_2 -> VLEDS
- D96 pad 2: GREEN_RIGHT_2 -> Net-(D88-Pad4)
- D96 pad 3: Segment_2-G_OUT -> GND
- D96 pad 4: BLUE_RIGHT_2 -> Net-(D95-Pad2)
- D97 pad 1: RED_RIGHT_2 -> VLEDS
- D97 pad 2: GREEN_RIGHT_2 -> Net-(D105-Pad4)
- D97 pad 3: Segment_2-D_OUT -> GND
- D97 pad 4: BLUE_RIGHT_2 -> Net-(D97-Pad4)
- D98 pad 1: RED_RIGHT_2 -> VLEDS
- D98 pad 2: GREEN_RIGHT_2 -> Net-(D97-Pad4)
- D98 pad 3: Segment_2-D_OUT -> GND
- D98 pad 4: BLUE_RIGHT_2 -> Net-(D171-Pad2)
- D99 pad 1: RED_RIGHT_2 -> VLEDS
- D99 pad 2: GREEN_RIGHT_2 -> Net-(D171-Pad4)
- D99 pad 3: Segment_2-A_OUT -> GND
- D99 pad 4: BLUE_RIGHT_2 -> Net-(D100-Pad2)
- J1 pad 1: +3V3 -> VDD
- J1 pad 6: SWO -> unconnected-(J1-Pad6)
- Q1 pad 2: +3V3 -> VBAT
- Q1 pad 3: Segment_2-A_OUT -> Net-(Q1-Pad3)
- Q2 pad 2: +3V3 -> VBUS
- Q2 pad 3: Segment_2-B_OUT -> VLEDS
- Q3 pad 2: +3V3 -> VBUS
- Q3 pad 3: Segment_2-C_OUT -> VLEDS_E
- Q4 pad 2: +3V3 -> VBUS
- Q4 pad 3: Segment_2-D_OUT -> Net-(BZ1-Pad1)
- R10 pad 1: Net-(Q21-Pad3) -> Net-(R10-Pad1)
- R10 pad 2: GREEN_LEFT_1 -> Net-(Q3-Pad1)
- R11 pad 1: Net-(Q22-Pad3) -> Net-(R11-Pad1)
- R11 pad 2: BLUE_LEFT_1 -> Net-(Q4-Pad1)
- R12 pad 1: Net-(D8-Pad1) -> VDD
- R12 pad 2: RED_BOTT_2 -> Net-(Q2-Pad1)
- R13 pad 1: Net-(D8-Pad2) -> VDD
- R13 pad 2: GREEN_BOTT_2 -> Net-(Q3-Pad1)
- R14 pad 1: Net-(D8-Pad4) -> VDD
- R14 pad 2: BLUE_BOTT_2 -> Net-(Q4-Pad1)
- R15 pad 1: Net-(D22-Pad1) -> R2_Data
- R15 pad 2: RED_BOTT_1 -> Net-(R15-Pad2)
- R16 pad 1: Net-(Q8-Pad3) -> R1_Data
- R16 pad 2: RED_BOTT_2 -> Net-(R16-Pad2)
- R17 pad 1: Net-(D22-Pad2) -> L1_Data
- R17 pad 2: GREEN_BOTT_1 -> Net-(R17-Pad2)
- R18 pad 1: Net-(Q9-Pad3) -> E1_Data
- R18 pad 2: RED_BOTT_1 -> Net-(R18-Pad2)
- R19 pad 1: Net-(D22-Pad4) -> Net-(R19-Pad1)
- R19 pad 2: BLUE_BOTT_1 -> L2_Data
- R2 pad 1: GND -> Net-(J2-PadB5)
- R2 pad 2: Net-(P1-PadA5) -> GND
- R3 pad 1: Net-(D24-Pad1) -> VBUS
- R3 pad 2: RED_BOTT_2 -> Net-(D1-Pad2)
- R4 pad 1: Net-(D24-Pad2) -> Net-(J3-Pad6)
- R4 pad 2: GREEN_BOTT_2 -> GND
- R5 pad 1: Net-(D24-Pad4) -> Net-(Q1-Pad3)
- R5 pad 2: BLUE_BOTT_2 -> Net-(R5-Pad2)
- R6 pad 1: Net-(D35-Pad1) -> Net-(R5-Pad2)
- R6 pad 2: RED_BOTT_2 -> GND
- R7 pad 1: Net-(D35-Pad2) -> VDD
- R7 pad 2: GREEN_BOTT_2 -> Net-(Q1-Pad1)
- R8 pad 1: Net-(D35-Pad4) -> Net-(R8-Pad1)
- R8 pad 2: BLUE_BOTT_2 -> Net-(Q1-Pad1)
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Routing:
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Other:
- outline, holes or cut-outs redrawn
- board text removed: "-"
- board text removed: "GND SWCLK GND SWDIO +3V3 SWO X X GND RST"
- board text removed: "Tag-Connect TC2050-IDC Programming Port"
